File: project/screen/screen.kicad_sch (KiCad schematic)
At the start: 34 parts, among them J1 Conn_01x06_Female, J2 USB_C_6pin, J3 Conn_01x02_Female, SW1 SW_DPDT_x2, SW2 SW_Push, SW3 SW_Push, U1 SPX3819M5-L-3-3, U2 ESP-12E, U3 TFT_1.3_12, U4 TP4056_[C16581]

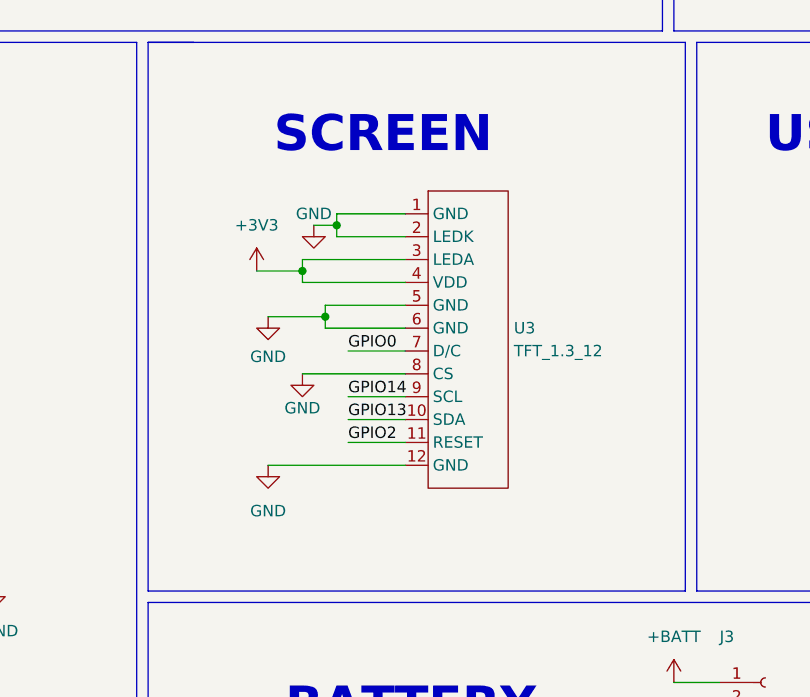
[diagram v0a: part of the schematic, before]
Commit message: update
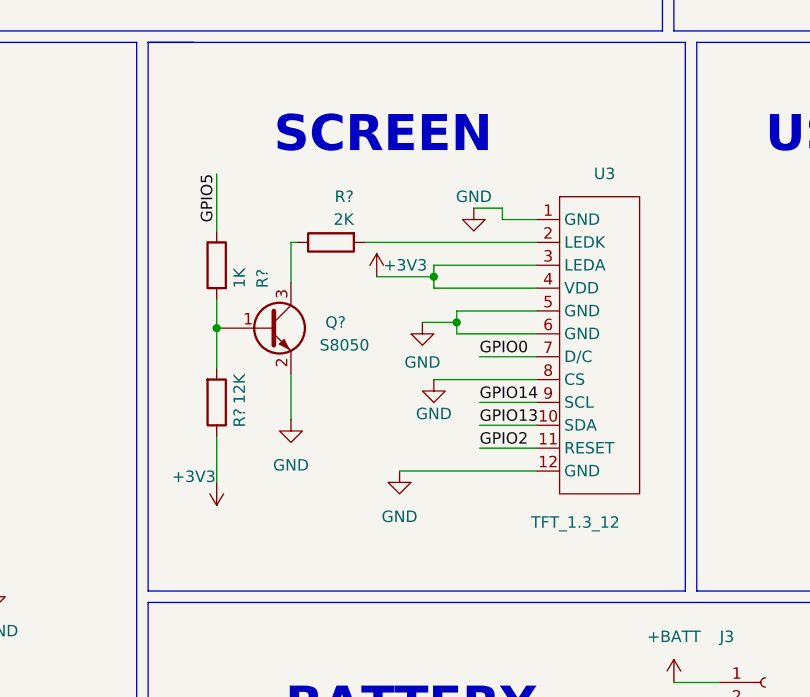
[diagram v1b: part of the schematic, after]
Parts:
- added Q?: S8050, symbol Device:Q_NPN_BEC
- added R?: 2K, Resistor_SMD:R_0402_1005Metric, symbol Device:R
- added R?: 1K, Resistor_SMD:R_0402_1005Metric, symbol Device:R
- added R?: 12K, Resistor_SMD:R_0402_1005Metric, symbol Device:R
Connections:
- net +3V3: now also R?.1
- net GND: now also Q?.2 (E); no longer U3.2 (LEDK)
- net GPIO5: now also R?.1
- new net: Q?.3 (C), R?.1
- new net: R?.2, U3.2 (LEDK)
- new net: Q?.1 (B), R?.2, R?.2
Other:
- moved on the sheet: U3
